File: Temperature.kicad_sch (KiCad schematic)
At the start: 29 parts, among them J3 Conn_01x24_Female, U8 LM321, U9 ADS7953SBDBT

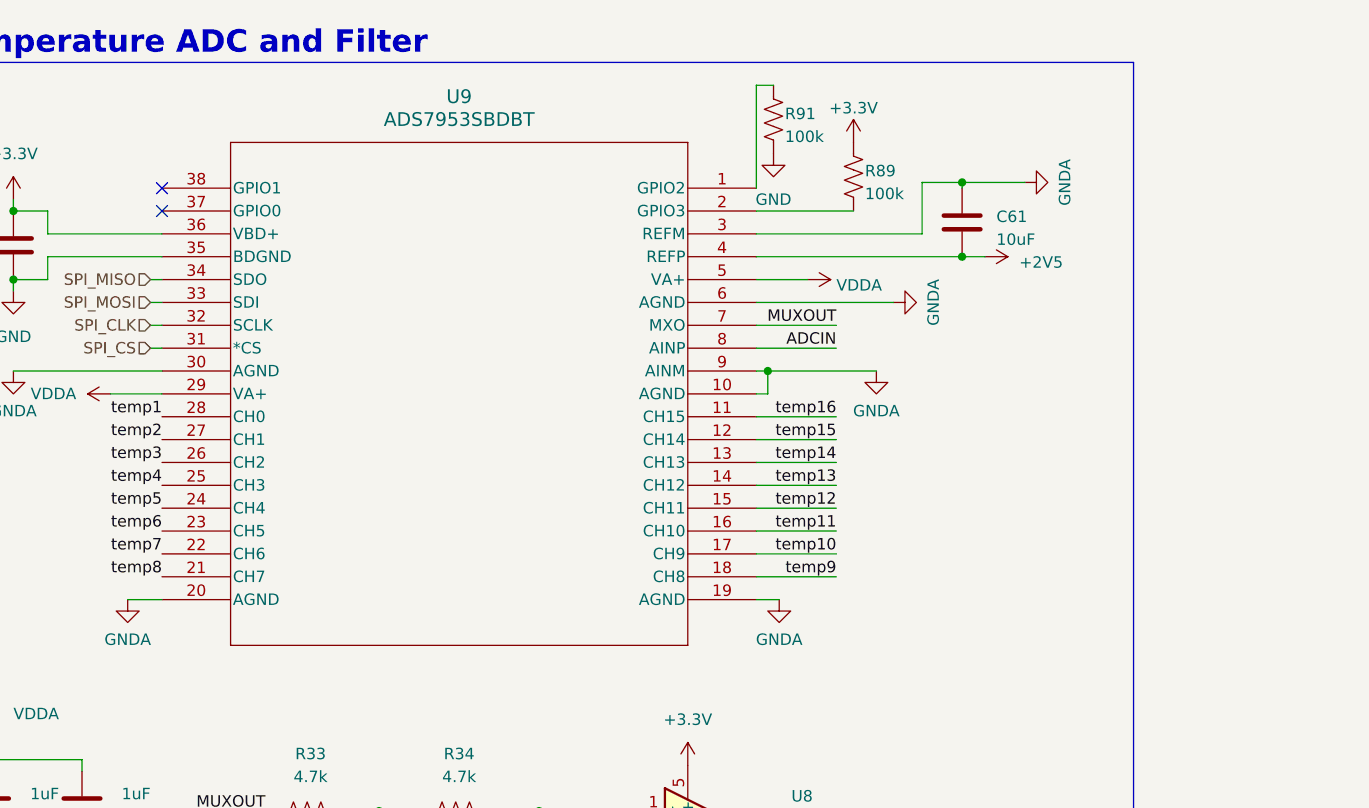
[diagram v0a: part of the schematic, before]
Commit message: layed out adc components, abt 75% done probably?
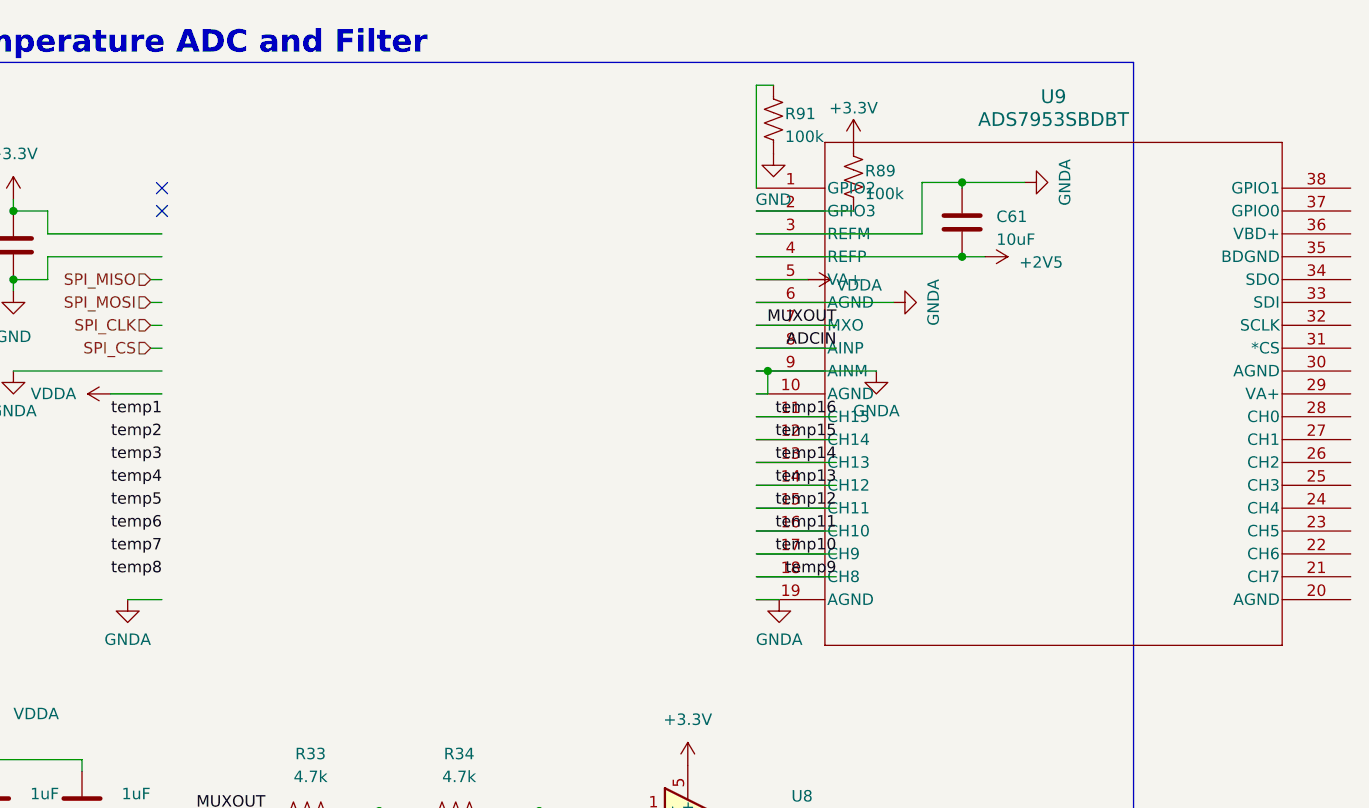
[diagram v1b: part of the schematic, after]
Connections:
- net +3.3V: no longer U9.36 (VBD+)
- net GND: no longer U9.35 (BDGND)
- net GNDA: no longer U9.20 (AGND), U9.30 (AGND)
- net SPI_CLK: no longer U9.32 (SCLK)
- net SPI_CS: no longer U9.31 (*CS)
- net SPI_MISO: no longer U9.34 (SDO)
- net SPI_MOSI: no longer U9.33 (SDI)
- net VDDA: no longer U9.29 (VA+)
- net temp1: no longer U9.28 (CH0)
- net temp2: no longer U9.27 (CH1)
- net temp3: no longer U9.26 (CH2)
- net temp4: no longer U9.25 (CH3)
- net temp5: no longer U9.24 (CH4)
- net temp6: no longer U9.23 (CH5)
- net temp7: no longer U9.22 (CH6)
- net temp8: no longer U9.21 (CH7)
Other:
- moved on the sheet: U9
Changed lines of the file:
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@@
     )
   )
-  (symbol (lib_id "utsvt-chips:ADS7953SBDBT") (at 237.49 31.75 0) (mirror y) (unit 1)
-    (in_bom yes) (on_board yes) (dnp no) (fields_autoplaced)
-    (property "Reference" "U9" (at 204.47 21.59 0)
+  (symbol (lib_id "utsvt-chips:ADS7953SBDBT") (at 237.49 31.75 0) (unit 1)
+    (in_bom yes) (on_board yes) (dnp no)
+    (property "Reference" "U9" (at 270.51 21.59 0)
       (effects (font (size 1.524 1.524)))
     )
-    (property "Value" "ADS7953SBDBT" (at 204.47 24.13 0)
+    (property "Value" "ADS7953SBDBT" (at 270.51 24.13 0)
       (effects (font (size 1.524 1.524)))
     )
